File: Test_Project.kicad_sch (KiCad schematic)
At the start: 67 parts, among them J2 Conn_01x02, J3 Conn_01x03, J4 Conn_01x03, J5 Conn_01x04, J6 Conn_01x04, Q1 NTTFS5C454NLTAG, Q2 NTTFS5C454NLTAG, Q3 NTTFS5C454NLTAG, Q4 NTTFS5C454NLTAG, Q5 Q_NMOS_DSG, U1 STM32L081KZTx, U2 MIC2132YML

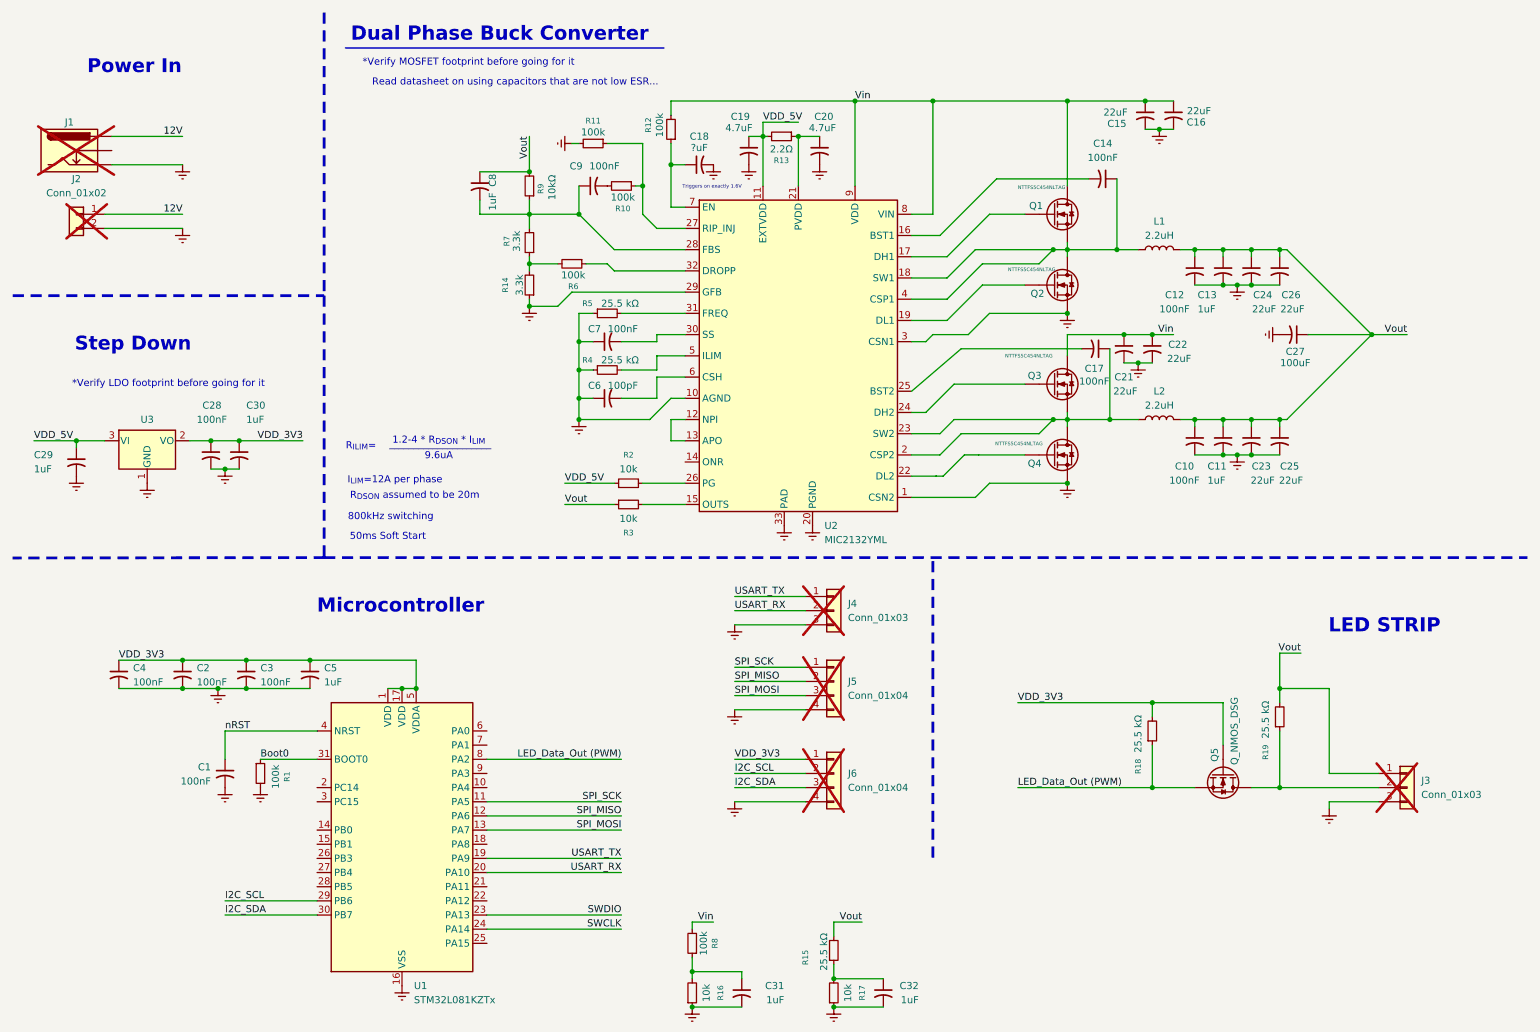
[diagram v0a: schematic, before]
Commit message: Started PCB layout
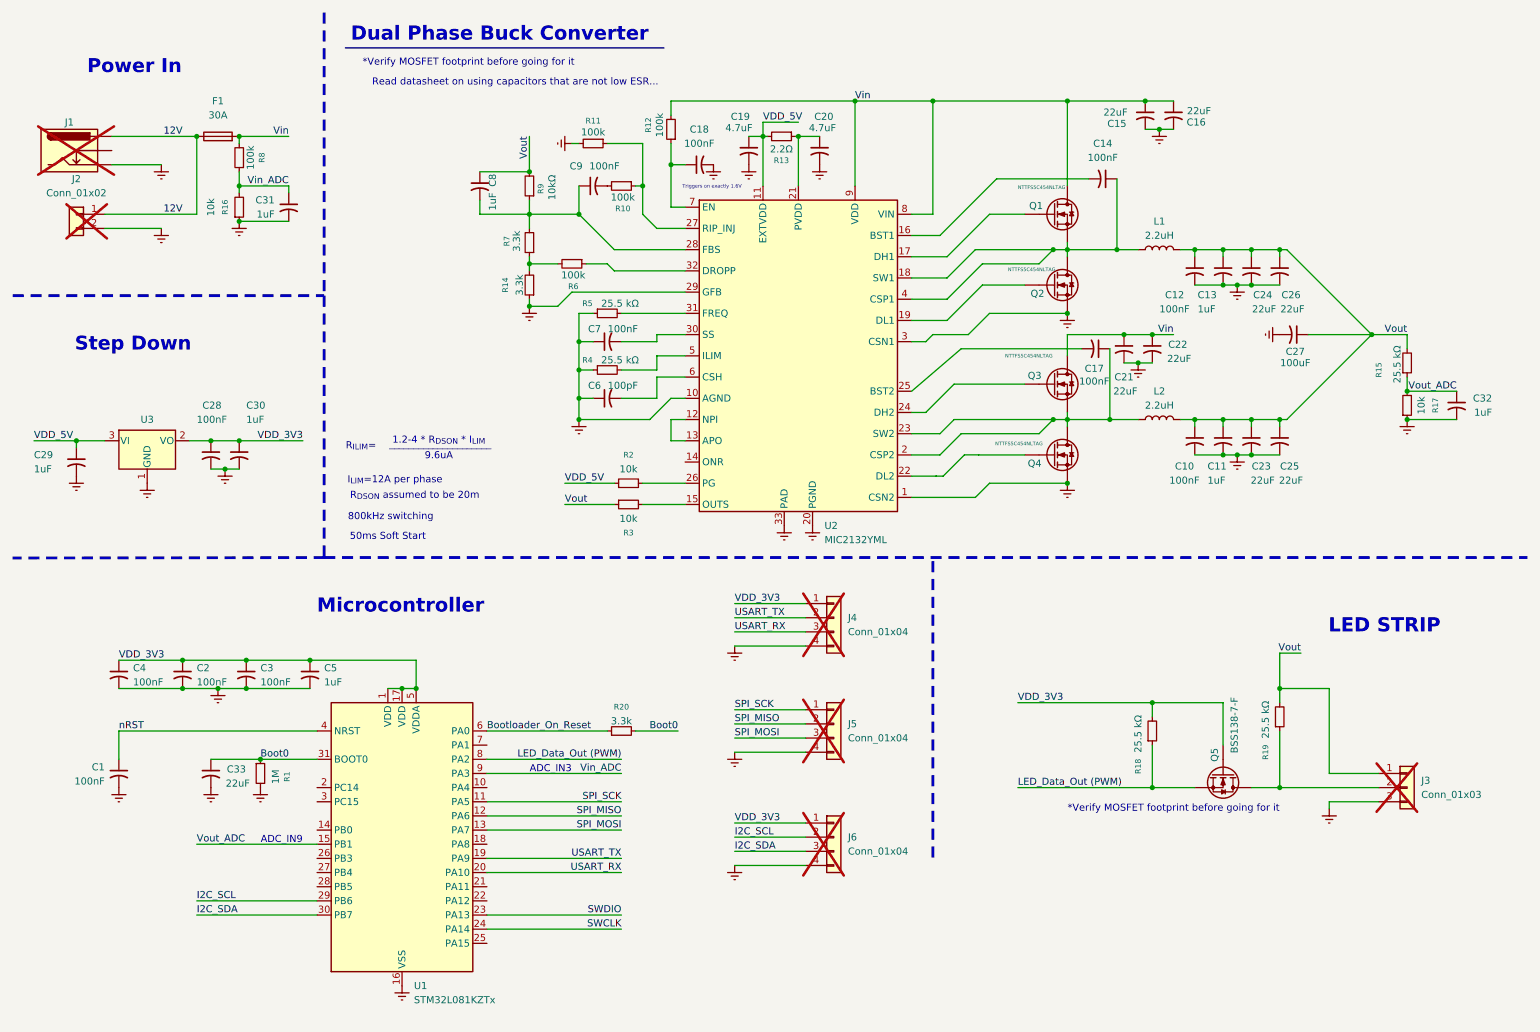
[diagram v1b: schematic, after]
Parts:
- removed J4: Conn_01x03, Connector_PinHeader_2.54mm:PinHeader_1x03_P2.54mm_Vertical, symbol Library:Conn_01x03
- added C33: 22uF, Capacitor_SMD:C_0805_2012Metric_Pad1.18x1.45mm_HandSolder, symbol Library:C_Small_US
- added F1: 0678L9300-02, Test_Project_Lib:Fuse - 0678L9300-02, symbol Device:Fuse
- added J4: Conn_01x04, Connector_PinHeader_2.54mm:PinHeader_1x04_P2.54mm_Vertical, symbol Library:Conn_01x04
- added R20: 3.3k, Resistor_SMD:R_0805_2012Metric_Pad1.20x1.40mm_HandSolder, symbol Library:R_Small
- C18: value ?uF -> 100nF
- L1, L2: footprint (none) -> Test_Project_Lib:SRP1265A
- Q1, Q2, Q3, Q4: footprint (none) -> Test_Project_Lib:NTTFS5C454NLTAG
- Q5: value Q_NMOS_DSG -> BSS138-7-F; footprint (none) -> Test_Project_Lib:BSS138-7-F
- R1: value 100k -> 1M
- U3: value ~ -> AP2127N-3.3TRG1
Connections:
- net 12V: now also F1.1
- net Boot0: now also C33.1, R20.2
- net USART_RX: now also J4.3 (Pin_3)
- net USART_TX: now also J4.2 (Pin_2)
- net VDD_3V3: now also J4.1 (Pin_1)
- net Vin: now also F1.2
- net GND: now reaches C2.2, C3.2, C4.2, C5.2
- net GND: now also C1.2, C10.2, C11.2, C12.2, C13.2, C15.2, C16.2, C18.2, C19.2, C20.2, C21.2, C22.2, C23.2, C24.2, C25.2, C26.2, C27.2, C28.2, C29.2, C30.2, C31.2, C32.2, C6.1, C7.1, J1.3, J2.2 (Pin_2), J3.3 (Pin_3), J5.4 (Pin_4), J6.4 (Pin_4), Q2.2 (S), Q4.2 (S), R1.2, R14.1, R16.1, R17.1, R4.1, R5.1, U1.16 (VSS), U1.32 (VSS), U2.1 (CSN2), U2.10 (AGND), U2.20 (PGND), U2.29 (GFB), U2.3 (CSN1), U2.33 (PAD), U3.1 (GND), C33.2, J4.4 (Pin_4)
- net Vout_ADC: now reaches C32.1, R15.1, R17.2
- net Vout_ADC: now also U1.15 (PB1)
- net Bootloader_On_Reset: now reaches U1.6 (PA0)
- net Bootloader_On_Reset: now also R20.1
- net Vin_ADC: now reaches U1.9 (PA3)
- net Vin_ADC: now also C31.1, R16.2, R8.1
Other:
- note added: "ADC_IN3"
- note added: "ADC_IN9"
- note removed: "*Verify LDO footprint before going for it"
- moved on the sheet: C1, C31, C32, J5, J6, R15, R16, R17, R8
